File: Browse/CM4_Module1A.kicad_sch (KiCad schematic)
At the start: 11 parts, among them Q2 50V

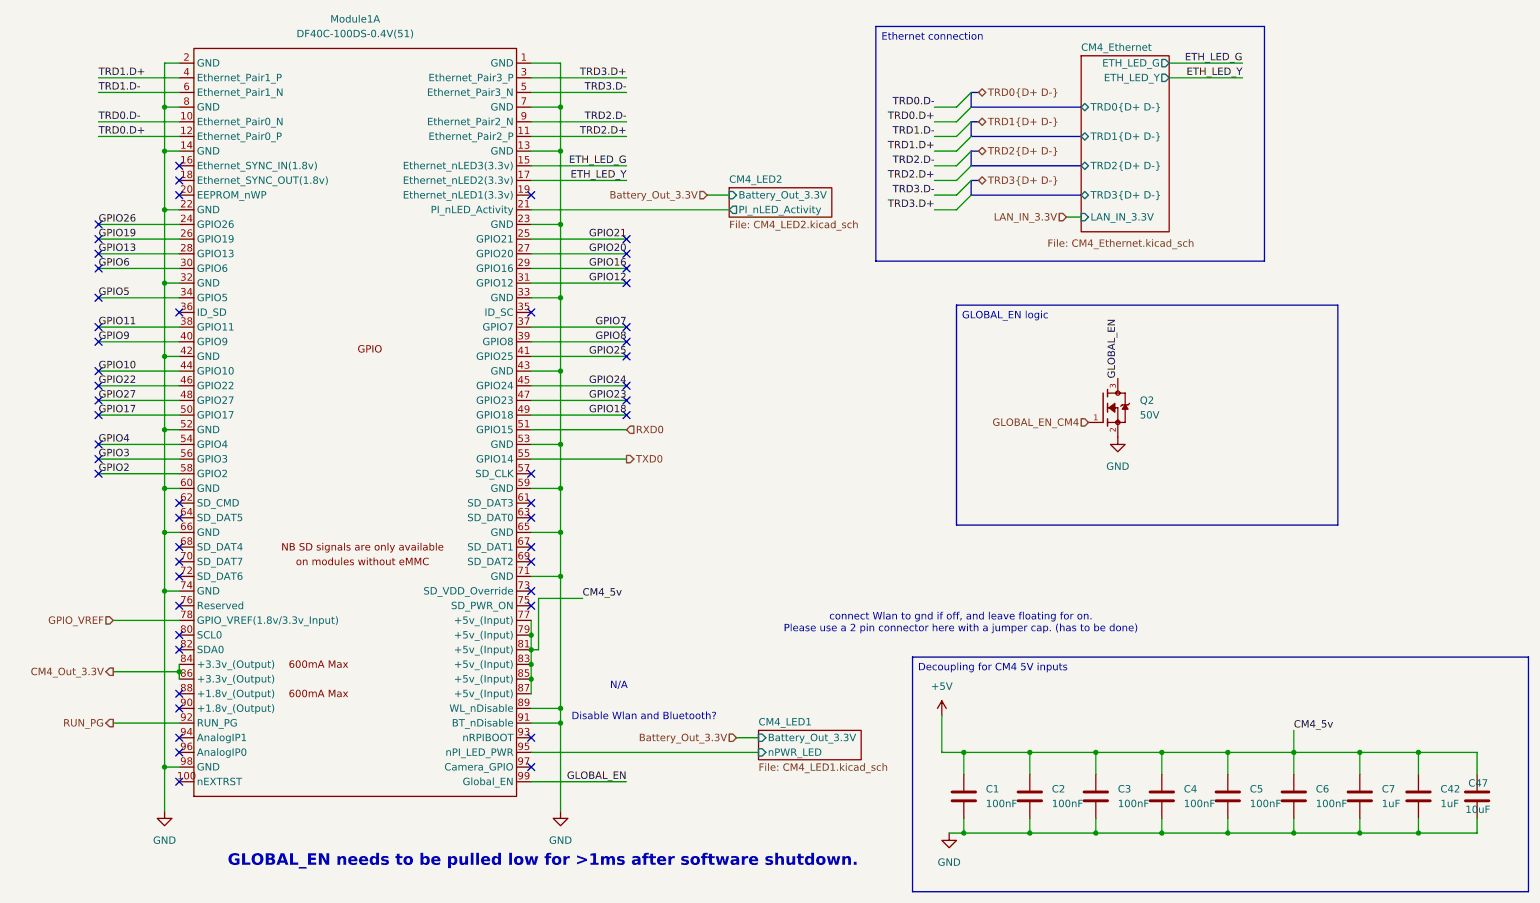
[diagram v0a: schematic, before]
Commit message: Deploying to gh-pages from @ Nautilus-UUV/nautilus-mainboard-PCB@5f5fdd9436d408a604bb268d740c0ac7ce1f5af5 🚀
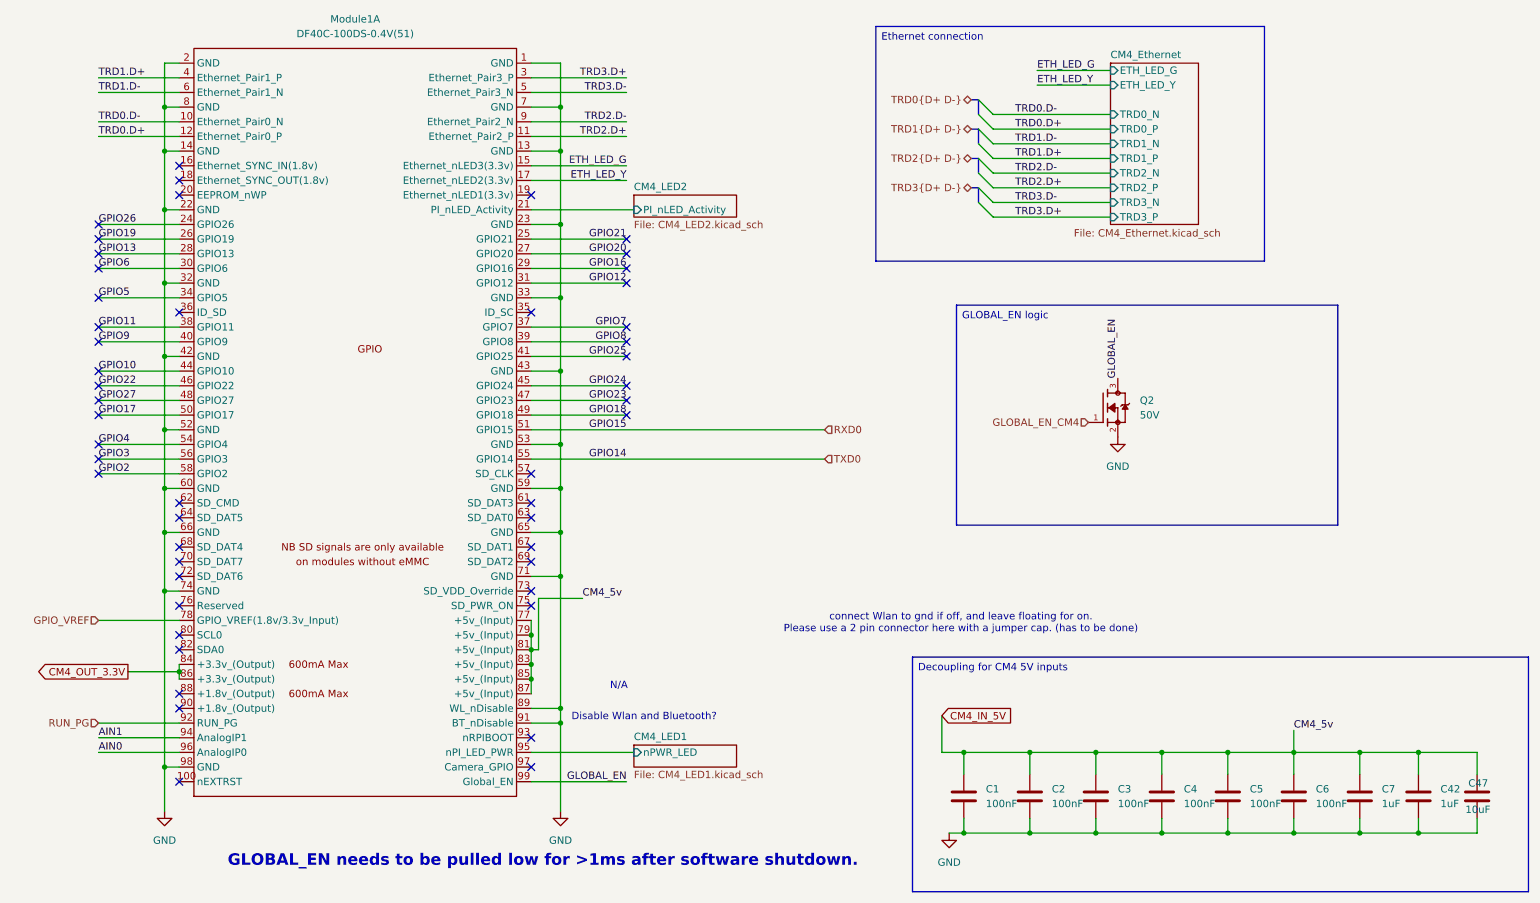
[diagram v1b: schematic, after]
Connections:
- net AIN1: now reaches Module1.94 (AnalogIP1)
- net AIN0: now reaches Module1.96 (AnalogIP0)
- net +5V renamed CM4_IN_5V
- net CM4_Out_3.3V renamed CM4_OUT_3.3V
- no-connect marks 52 -> 50
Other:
- sheet CM4_Ethernet ports: added TRD0_N, TRD0_P, TRD1_N, TRD1_P, TRD2_N, TRD2_P, TRD3_N, TRD3_P; removed LAN_IN_3.3V, TRD0{D+ D-}, TRD1{D+ D-}, TRD2{D+ D-}, TRD3{D+ D-}
- sheet CM4_LED1 ports: added none; removed Battery_Out_3.3V
- sheet CM4_LED2 ports: added none; removed Battery_Out_3.3V
- company: Davide -> (none)
- title: Nautilus_Mainboard -> (none)
